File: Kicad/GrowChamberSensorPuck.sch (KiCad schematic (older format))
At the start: 13 parts, among them P1 CONN_01X07, U1 Si7006, U2 CCS811

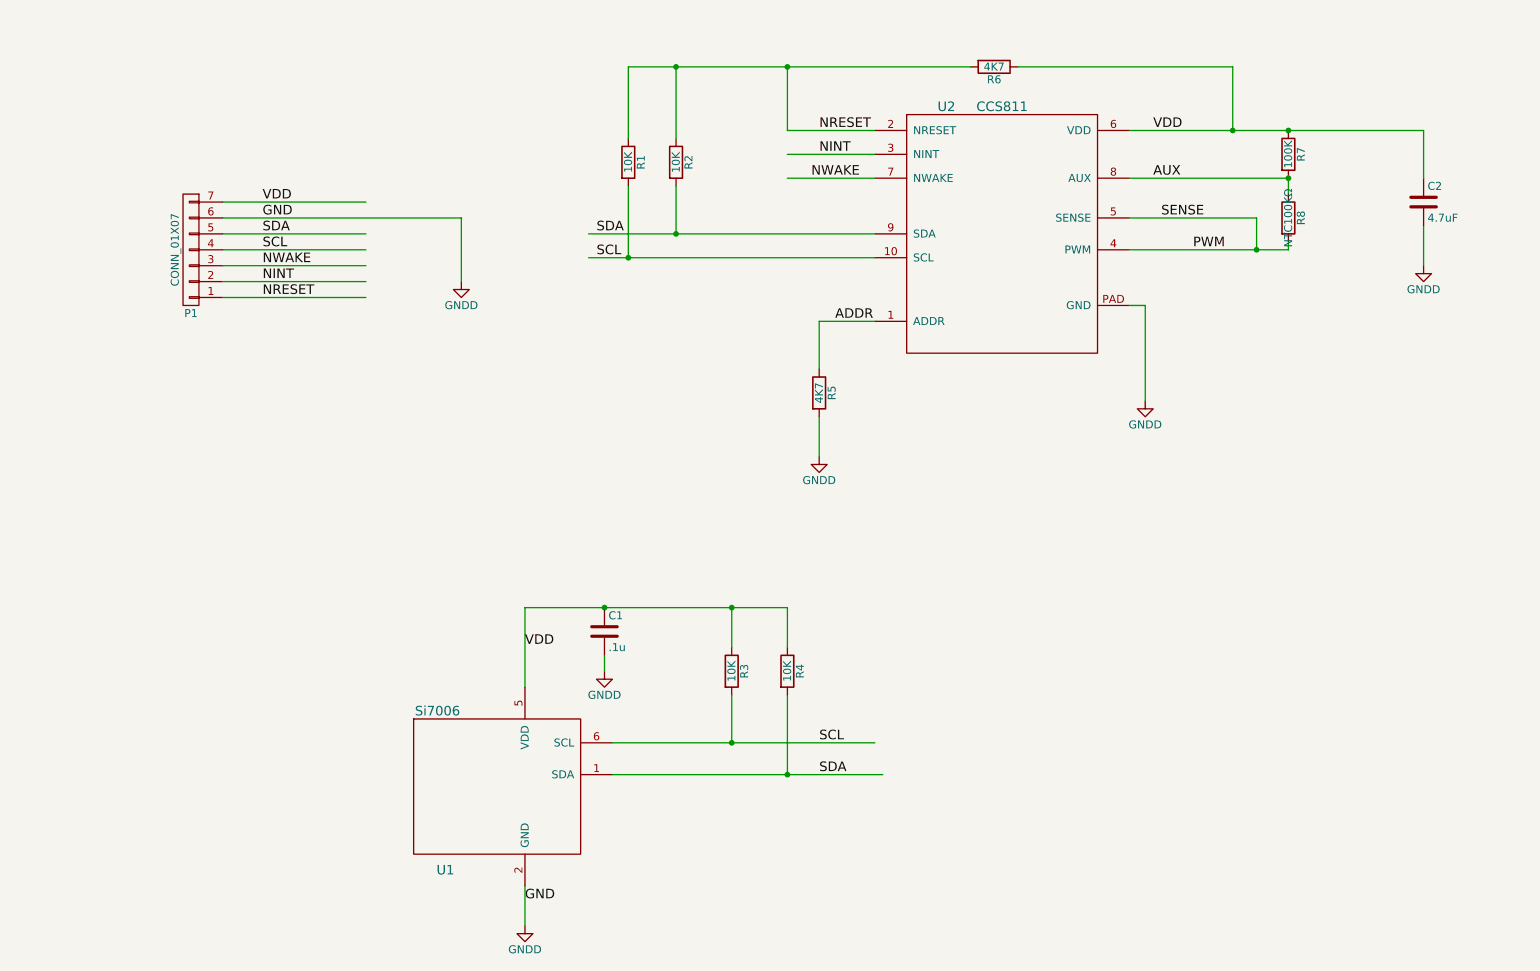
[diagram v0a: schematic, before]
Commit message: evolved Grow Sensor Puck schematic
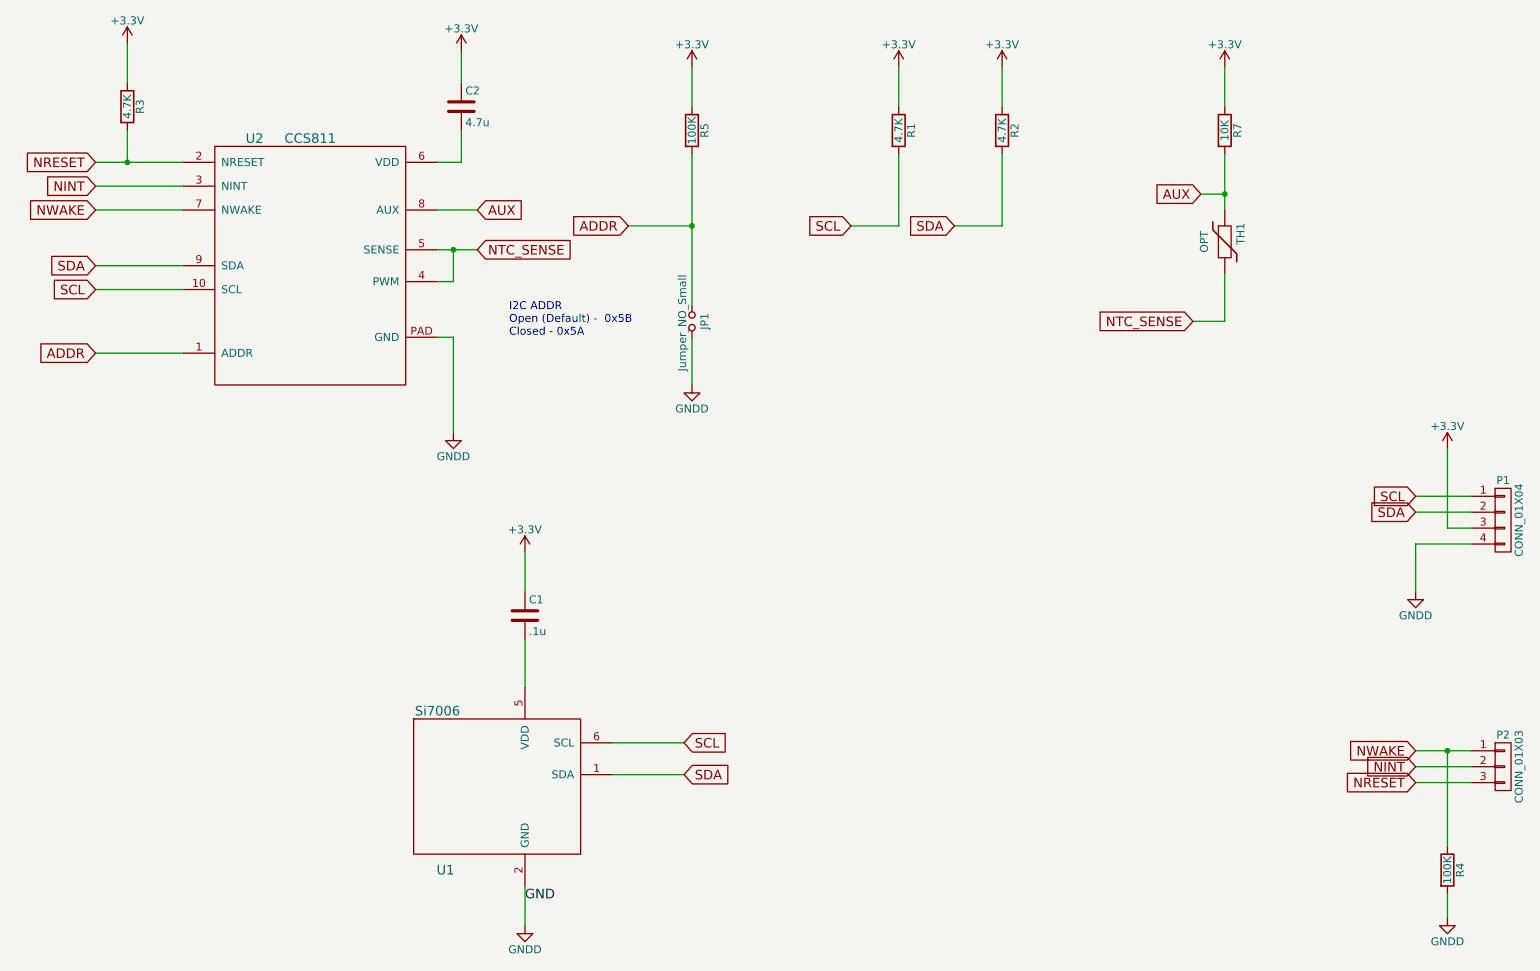
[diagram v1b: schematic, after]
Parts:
- removed P1: CONN_01X07, symbol CONN_01X07
- removed R6: 4K7, Capacitors_SMD:C_0805_HandSoldering, symbol R
- removed R8: NTC100KΩ, symbol R
- added JP1: Jumper_NO_Small, symbol Jumper_NO_Small
- added P1: CONN_01X04, symbol CONN_01X04
- added P2: CONN_01X03, symbol CONN_01X03
- added TH1: OPT, symbol Thermistor
- C2: value 4.7uF -> 4.7u
- R1, R2, R3: value 10K -> 4.7K
- R4: value 10K -> 100K
- R5: value 4K7 -> 100K
- R7: value 100K -> 10K
- U1: footprint (none) -> TheLeafSpa:Si7006
- U2: footprint (none) -> TheLeafSpa:CCS811
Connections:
- net labels added: +3.3V, NTC_SENSE
- net labels removed: PWM, SENSE, VDD
- wire segments 45 -> 48
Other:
- note added: "I2C ADDR\nOpen (Default) - 0x5B\nClosed - 0x5A"
- moved on the sheet: C1, C2, R1, R5, R7, U2
